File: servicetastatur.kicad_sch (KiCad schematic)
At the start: 21 parts, among them J1 Conn_02x08_Odd_Even, J2 Conn_01x06_Socket, U1 AT24CS16-SSHM, U2 TL7705A, U3 74HC165, U4 74HC00, U5 MC34063AP, U6 27C128, Y1 Crystal

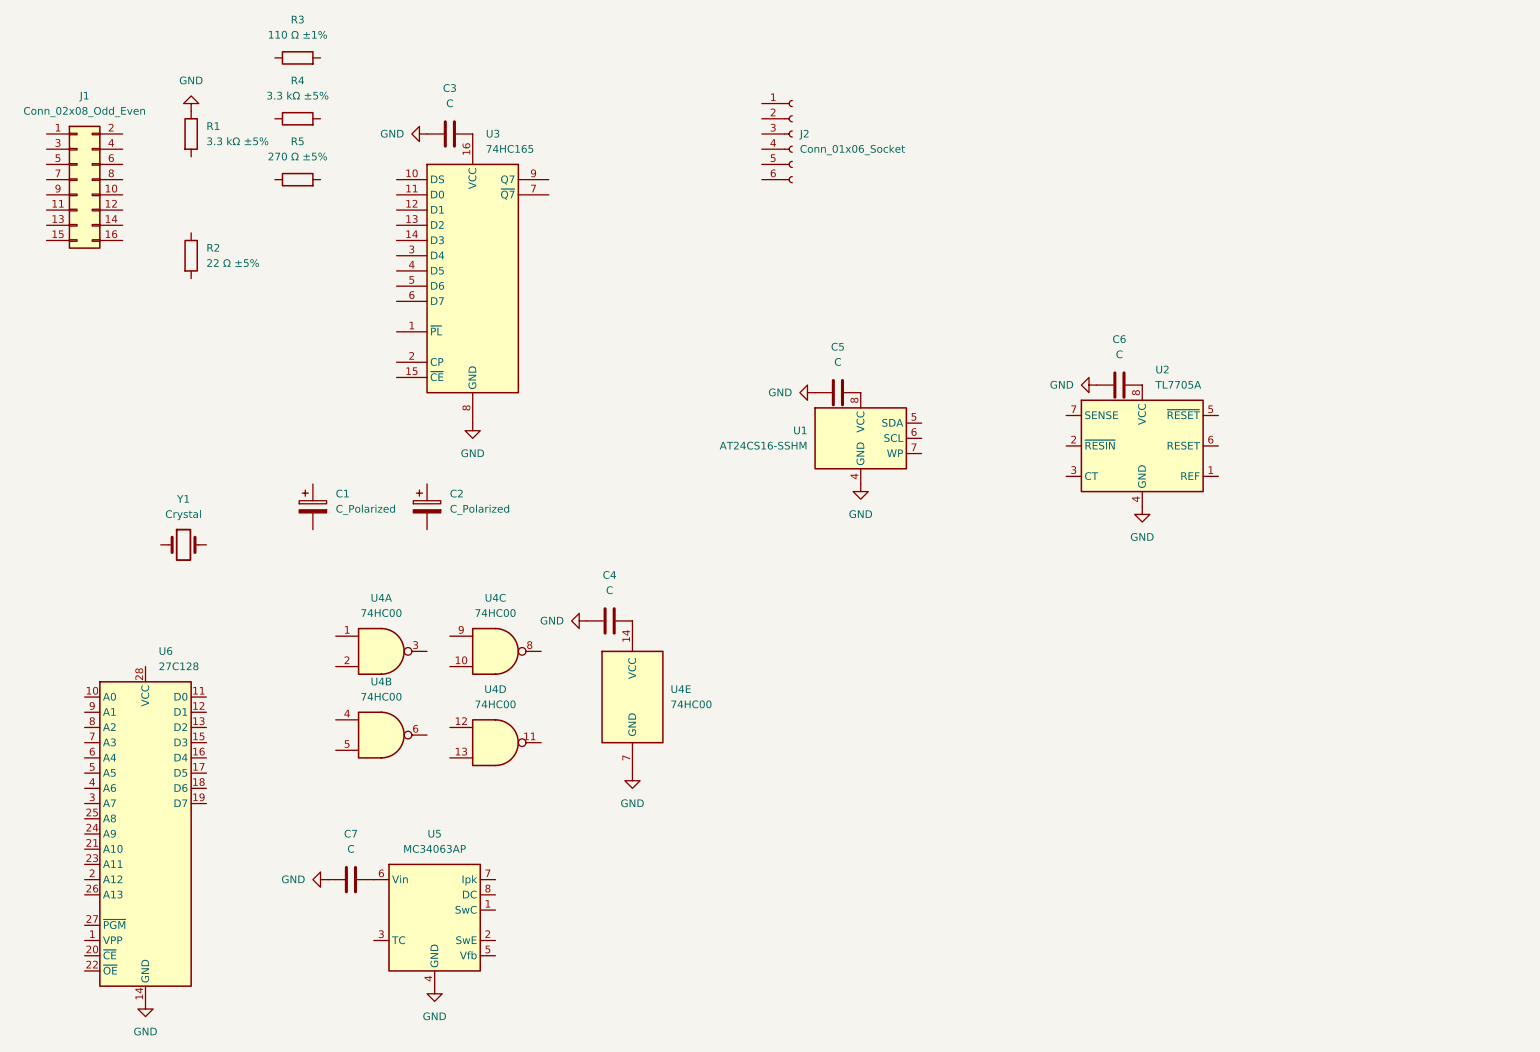
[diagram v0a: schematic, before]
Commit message: CPU
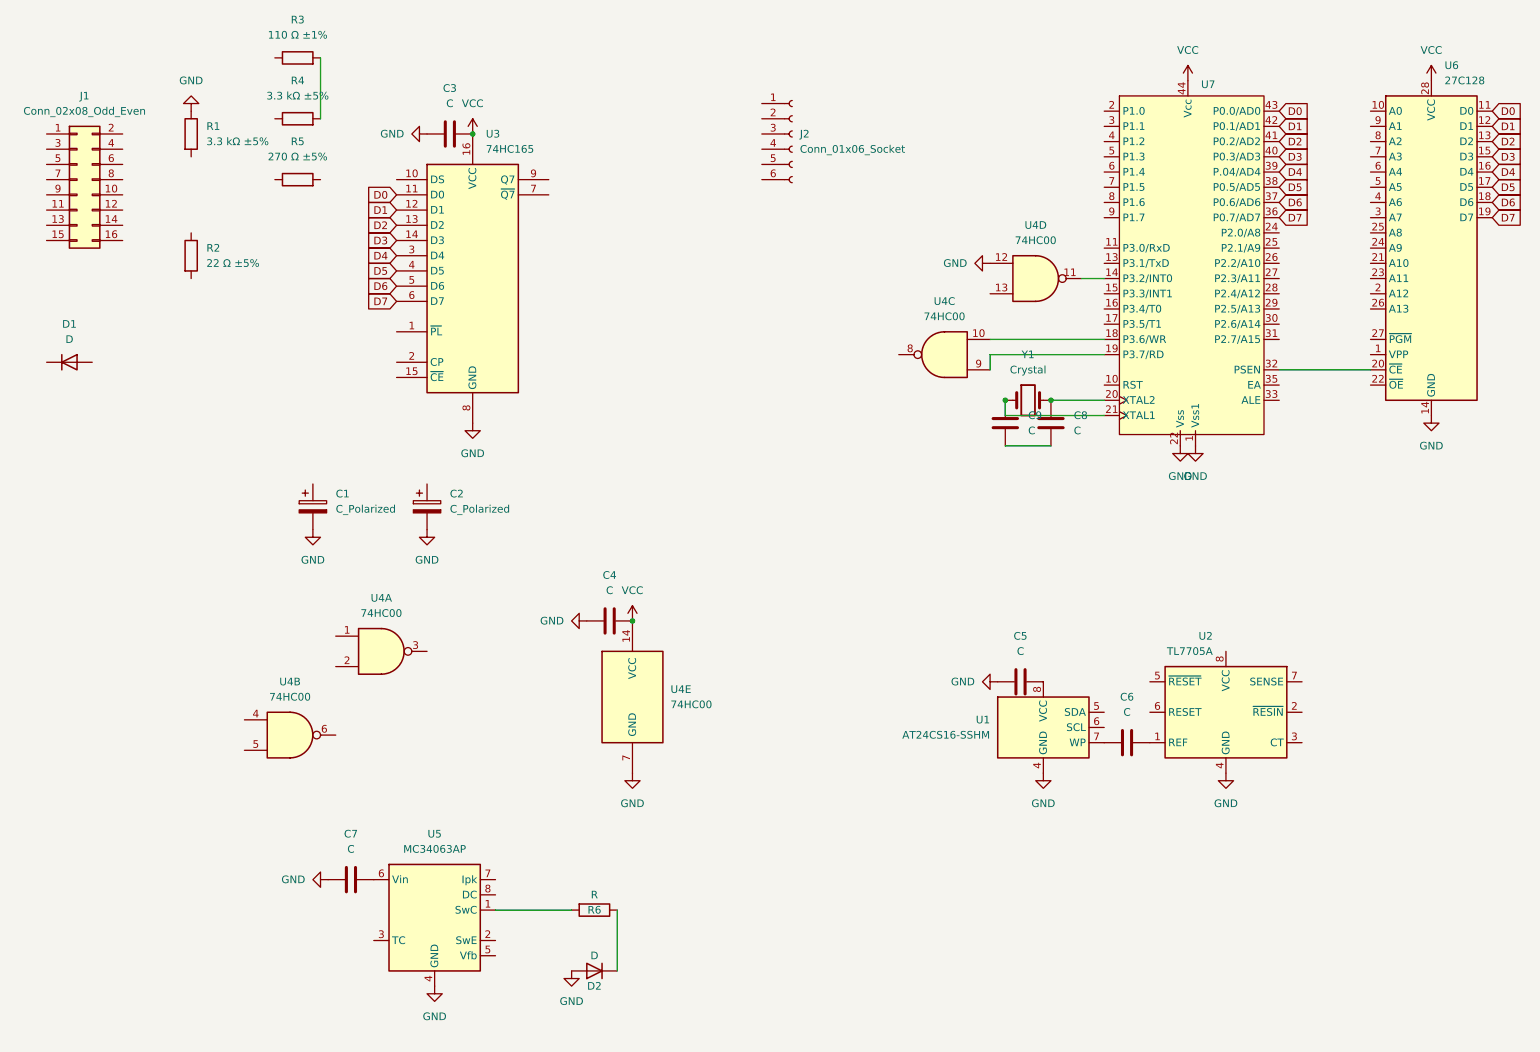
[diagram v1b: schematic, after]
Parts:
- added C8, C9: C, Capacitor_THT:CP_Radial_Tantal_D4.5mm_P2.50mm, symbol Device:C
- added D1, D2: D, Diode_THT:D_DO-15_P15.24mm_Horizontal, symbol Device:D
- added R6: R, Resistor_THT:R_Axial_DIN0414_L11.9mm_D4.5mm_P15.24mm_Horizontal, symbol Device:R
- added U7: ~, Package_LCC:PLCC-44_THT-Socket, symbol MCU_Atmel:TS80C31
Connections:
- net GND: now also C1.2, C2.2, U4.12, D2.2 (A), U7.1 (Vss1), U7.22 (Vss); no longer C6.1
- net at U4.10: now also U7.18 (P3.6/WR)
- net at U4.9: now also U7.19 (P3.7/RD)
- net VCC: now reaches C4.2, U4.14 (VCC)
- net VCC: now also C3.2, U3.16 (VCC), U6.28 (VCC), U7.44 (Vcc)
- net at R4.2: now also R3.2
- net D0: now reaches U6.11 (D0)
- net D0: now also U3.11 (D0), U7.43 (P0.0/AD0)
- net D1: now reaches U6.12 (D1)
- net D1: now also U3.12 (D1), U7.42 (P0.1/AD1)
- net D2: now reaches U6.13 (D2)
- net D2: now also U3.13 (D2), U7.41 (P0.2/AD2)
- net D3: now reaches U6.15 (D3)
- net D3: now also U3.14 (D3), U7.40 (P0.3/AD3)
- net D4: now reaches U6.16 (D4)
- net D4: now also U3.3 (D4), U7.39 (P.04/AD4)
- net D5: now reaches U6.17 (D5)
- net D5: now also U3.4 (D5), U7.38 (P0.5/AD5)
- net D6: now reaches U6.18 (D6)
- net D6: now also U3.5 (D6), U7.37 (P0.6/AD6)
- net D7: now reaches U6.19 (D7)
- net D7: now also U3.6 (D7), U7.36 (P0.7/AD7)
- net at U6.20 (~{CE}): now also U7.32 (PSEN)
- net at Y1.1: now also C9.2, U7.21 (XTAL1)
- net at Y1.2: now also C8.2, U7.20 (XTAL2)
- net at U4.11: now also U7.14 (P3.2/INT0)
- net at U1.7 (WP): now also C6.1
- net at U2.1 (REF): now also C6.2
- net at U2.8 (VCC): no longer C6.2
- net at U5.1 (SwC): now also R6.2
- new net: D2.1 (K), R6.1
- new net: C8.1, C9.1
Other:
- moved on the sheet: C5, C6, U1, U2, U4B, U4C, U4D, U6, Y1
